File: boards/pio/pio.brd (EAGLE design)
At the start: 160 x 100 mm, 9 parts

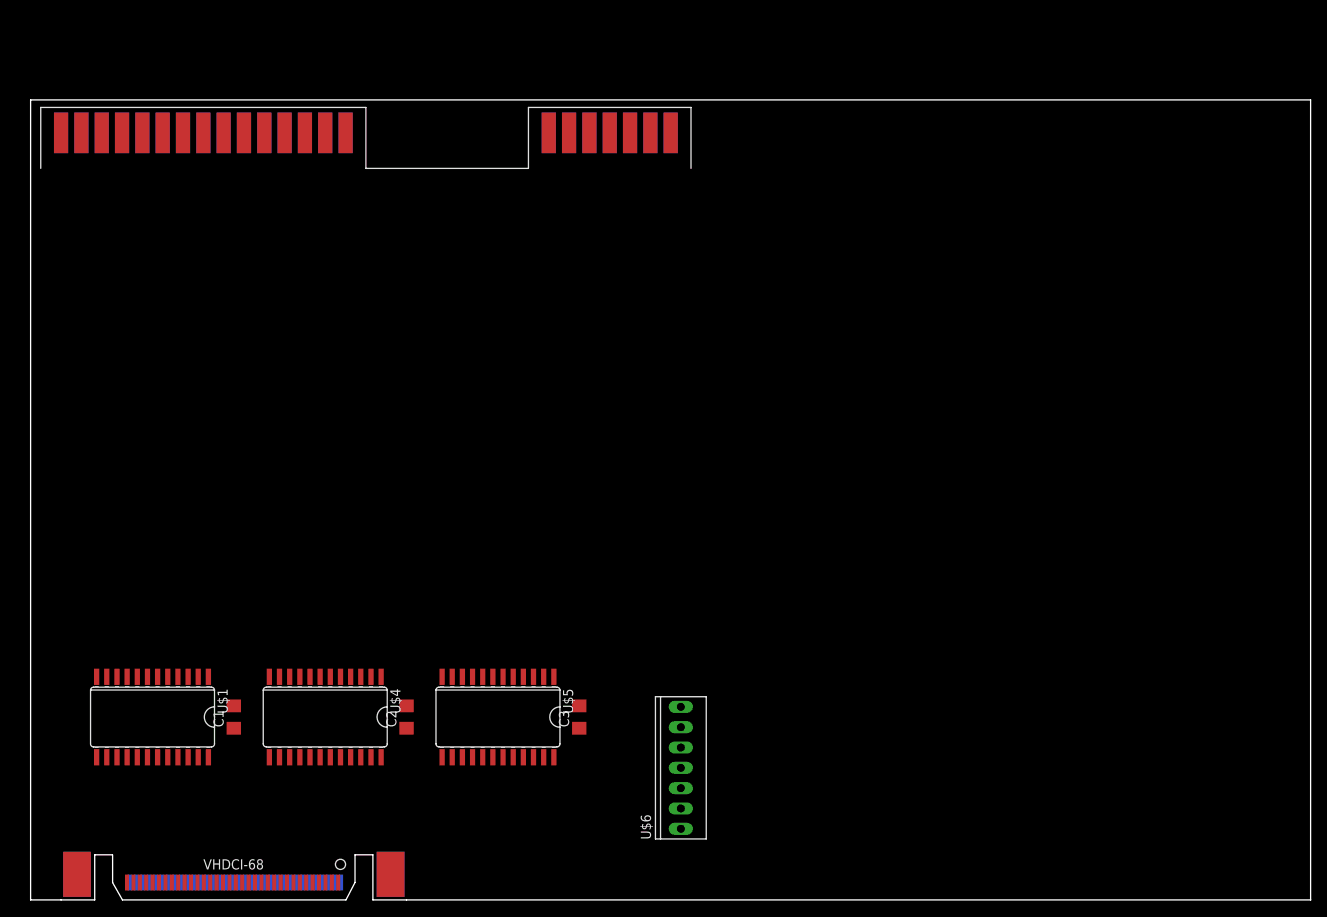
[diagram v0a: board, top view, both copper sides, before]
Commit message: Version of PIO to send off for manufacture
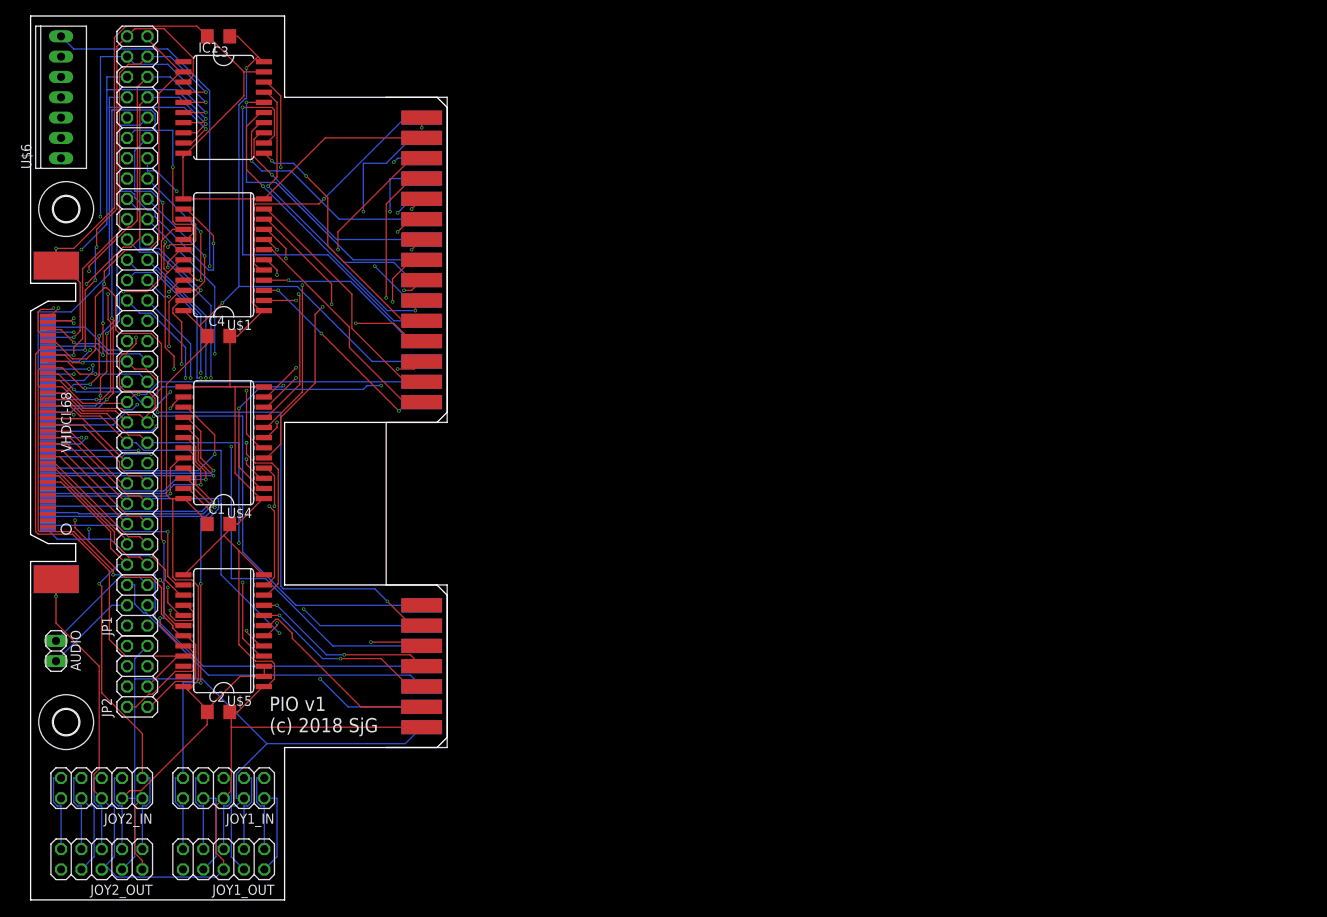
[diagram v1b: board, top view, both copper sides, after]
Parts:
- added AUDIO: (no value), pinhead:1X02
- added C4: 0.1uF, rcl:C1206
- added H1, H2: MOUNT-HOLE3.2, holes:3,2
- added IC1: 74AC245DW, 74xx-eu:SO20W
- added JOY1_IN, JOY1_OUT, JOY2_IN, JOY2_OUT: (no value), pinhead:2X05
- added JP1: (no value), pinhead:2X30
- added JP2: (no value), pinhead:2X04
- moved U$6 114.1 mm to (3.81, 100.3)
- moved C3 96.3 mm to (23.5, 108.0), turned to 180 degrees
- moved U$3 64.9 mm to (0.00, 59.7), turned to 270 degrees
- moved U$1 58.5 mm to (24.1, 80.6), turned to 90 degrees
- moved U$2 44.1 mm to (44.5, 100.3), turned to 270 degrees
- moved U$4 36.6 mm to (24.1, 57.1), turned to 90 degrees
- moved U$5 35.9 mm to (24.1, 33.7), turned to 90 degrees
- moved C1 24.2 mm to (23.5, 47.0), turned to 0 degrees
- moved C2 23.5 mm to (23.5, 23.5), turned to 0 degrees
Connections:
- removed net N$12: U$1.19, U$3.P53
- removed net N$13: U$1.20, U$3.P52
- removed net N$14: U$1.21, U$3.P51
- removed net N$15: U$1.14, U$3.P58
- removed net N$16: U$1.15, U$3.P57
- removed net N$17: U$1.16, U$3.P56
- removed net N$18: U$1.17, U$3.P55
- removed net N$19: U$1.18, U$3.P54
- removed net N$2: U$2.P$35, U$3.P68
- removed net N$20: U$1.22, U$3.P50
- removed net N$21: U$1.23, U$3.P49
- removed net N$32: U$3.P48, U$4.14
- removed net N$33: U$3.P47, U$4.15
- removed net N$34: U$3.P46, U$4.16
- removed net N$35: U$3.P45, U$4.17
- removed net N$36: U$3.P44, U$4.18
- removed net N$37: U$3.P43, U$4.19
- removed net N$38: U$3.P42, U$4.20
- removed net N$39: U$3.P41, U$4.21
- removed net N$40: U$3.P40, U$4.22
- removed net N$41: U$3.P39, U$4.23
- removed net N$50: U$3.P38, U$5.14
- removed net N$51: U$3.P37, U$5.15
- removed net N$52: U$3.P36, U$5.16
- removed net N$53: U$3.P35, U$5.17
- removed net N$54: U$3.P34, U$5.18
- removed net N$55: U$3.P33, U$5.19
- removed net N$56: U$3.P32, U$5.20
- removed net N$57: U$3.P31, U$5.21
- new net A0: JP1.44, U$1.23, U$3.P47
- new net A1: JP1.41, U$3.P46, U$4.14
- new net A10: JP1.34, U$3.P37, U$4.23
- new net A11: JP1.31, U$3.P36, U$5.14
- new net A12: JP1.32, U$3.P35, U$5.15
- new net A13: JP1.29, U$3.P34, U$5.16
- new net A14: JP1.30, U$3.P33, U$5.17
- new net A15: JP1.27, U$3.P32, U$5.18
- new net A2: JP1.42, U$3.P45, U$4.15
- new net A3: JP1.39, U$3.P44, U$4.16
- new net A4: JP1.40, U$3.P43, U$4.17
- new net A5: JP1.37, U$3.P42, U$4.18
- new net A6: JP1.38, U$3.P41, U$4.19
- new net A7: JP1.35, U$3.P40, U$4.20
- new net A8: JP1.36, U$3.P39, U$4.21
- new net A9: JP1.33, U$3.P38, U$4.22
- new net AUDIO: JP1.6, U$2.P$35, U$3.P66
- new net AUDIO_L: AUDIO.2, JP1.4, U$3.P67
- new net AUDIO_R: AUDIO.1, JP1.5, U$3.P68
- new net B02: JP1.47, U$1.18, U$3.P52
- new net CCTL: JP1.43, U$1.22, U$3.P48
- new net COMMAND: JP2.1, U$3.P31, U$5.19
- new net D0: IC1.2, JP1.59, U$3.P64
- new net D1: IC1.3, JP1.60, U$3.P63
- new net D1XX: JP1.50, U$1.17, U$3.P53
- new net D2: IC1.4, JP1.57, U$3.P62
- new net D3: IC1.5, JP1.58, U$3.P61
- new net D4: IC1.6, JP1.55, U$3.P60
- new net D5: IC1.7, JP1.56, U$3.P59
- new net D6: IC1.8, JP1.53, U$3.P58
- new net D7: IC1.9, JP1.54, U$3.P57
- new net DATA_OUT: JP2.2, U$3.P30, U$5.20
- new net G_IN0: JP1.3
- new net G_IN1: JP1.2
- new net G_IN2: JP1.1
- new net HALT: JP1.52, U$1.15, U$3.P55
- new net J1_1: JOY1_IN.1, JOY1_OUT.1, JP1.19, U$3.P21
- new net J1_2: JOY1_IN.2, JOY1_OUT.2, JP1.20, U$3.P20
- new net J1_3: JOY1_IN.3, JOY1_OUT.3, JP1.17, U$3.P19
- new net J1_4: JOY1_IN.5, JOY1_OUT.5, JP1.18, U$3.P18
- new net J1_5: JOY1_IN.7, JOY1_OUT.7, JP1.15, U$3.P17
- new net J1_A1: JOY1_IN.8, JOY1_OUT.8, JP1.16, U$3.P16
- new net J1_A2: JOY1_IN.9, JOY1_OUT.9, JP1.13, U$3.P15
- new net J2_1: JOY2_IN.1, JOY2_OUT.1, JP1.8, U$3.P8
- new net J2_2: JOY2_IN.2, JOY2_OUT.2, JP1.7, U$3.P9
- new net J2_3: JOY2_IN.3, JOY2_OUT.3, JP1.10, U$3.P10
- new net J2_4: JOY2_IN.5, JOY2_OUT.5, JP1.9, U$3.P11
- new net J2_5: JOY2_IN.7, JOY2_OUT.7, JP1.12, U$3.P12
- new net J2_A1: JOY2_IN.8, JOY2_OUT.8, JP1.11, U$3.P13
- new net J2_A2: JOY2_IN.9, JOY2_OUT.9, JP1.14, U$3.P14
- new net MTR_CTRL: JP2.3, U$3.P29, U$5.21
- new net N$67: IC1.11, U$2.P$11
- new net N$68: IC1.12, U$2.P$26
- new net N$69: IC1.13, U$2.P$22
- new net N$70: IC1.14, U$2.P$21
- new net N$71: IC1.15, U$2.P$10
- new net N$72: IC1.16, U$2.P$23
- new net N$73: IC1.17, U$2.P$24
- new net N$74: IC1.18, U$2.P$25
- new net REF: JP1.48, U$1.19, U$3.P51
- new net RST: JP1.49, U$1.16, U$3.P54
- new net RW: JP1.51, U$1.14, U$3.P56
- new net S4: JP1.45, U$1.20, U$3.P50
- new net S5: JP1.46, U$1.21, U$3.P49
- net !EXSEL!: now also JP1.25
- net !IRQ!: now also JP1.28, U$3.P28; no longer U$3.P26
- net !MPD!: now also JP1.26, U$3.P26; no longer U$3.P28
- net +5V: now also C4.1, IC1.20, JOY1_IN.4, JOY1_OUT.4, JOY2_IN.4, JOY2_OUT.4, JP2.7
- net GND: now also C4.2, IC1.10, IC1.19, JOY1_IN.6, JOY1_OUT.6, JOY2_IN.6, JOY2_OUT.6, U$3.P65; no longer U$3.P67
- net RD4: now also JP1.23, U$3.P25; no longer U$3.P30
- net RD5: now also JP1.24, U$3.P24; no longer U$3.P29
- net SIO_CLK_IN: now also JP1.22, U$3.P22; no longer U$3.P25
- net SIO_DATA_IN: now also JP1.21, U$3.P23; no longer U$3.P24
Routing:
- net GND: track 0.00 -> 329.3 mm, vias 0 -> 3
- net +5V: track 0.00 -> 251.3 mm, vias 0 -> 2
- net N$42: track 0.00 -> 93.0 mm, vias 0 -> 1
- net !MPD!: track 0.00 -> 91.2 mm, vias 0 -> 2
- net N$43: track 0.00 -> 86.1 mm, vias 0 -> 1
- net J1_2: track 0.00 -> 82.4 mm, vias 0 -> 1
- net DATA_OUT: track 0.00 -> 81.8 mm, vias 0 -> 2
- net AUDIO: track 0.00 -> 81.5 mm, vias 0 -> 1
- net N$44: track 0.00 -> 80.8 mm, vias 0 -> 1
- net J1_1: track 0.00 -> 79.9 mm, vias 0 -> 1
- net SIO_CLK_IN: track 0.00 -> 79.4 mm, vias 0 -> 1
- net !IRQ!: track 0.00 -> 76.0 mm, vias 0 -> 3
- net D1XX: track 0.00 -> 75.2 mm, vias 0 -> 3
- net N$3: track 0.00 -> 74.9 mm, vias 0 -> 2
- net J1_A2: track 0.00 -> 74.2 mm, vias 0 -> 2
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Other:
- board size 160 x 100 mm -> 52.1 x 110.5 mm
- board text added: "PIO v1 (c) 2018 SjG"

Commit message: Ok, belay that last. *This* is the one to go to the fab.
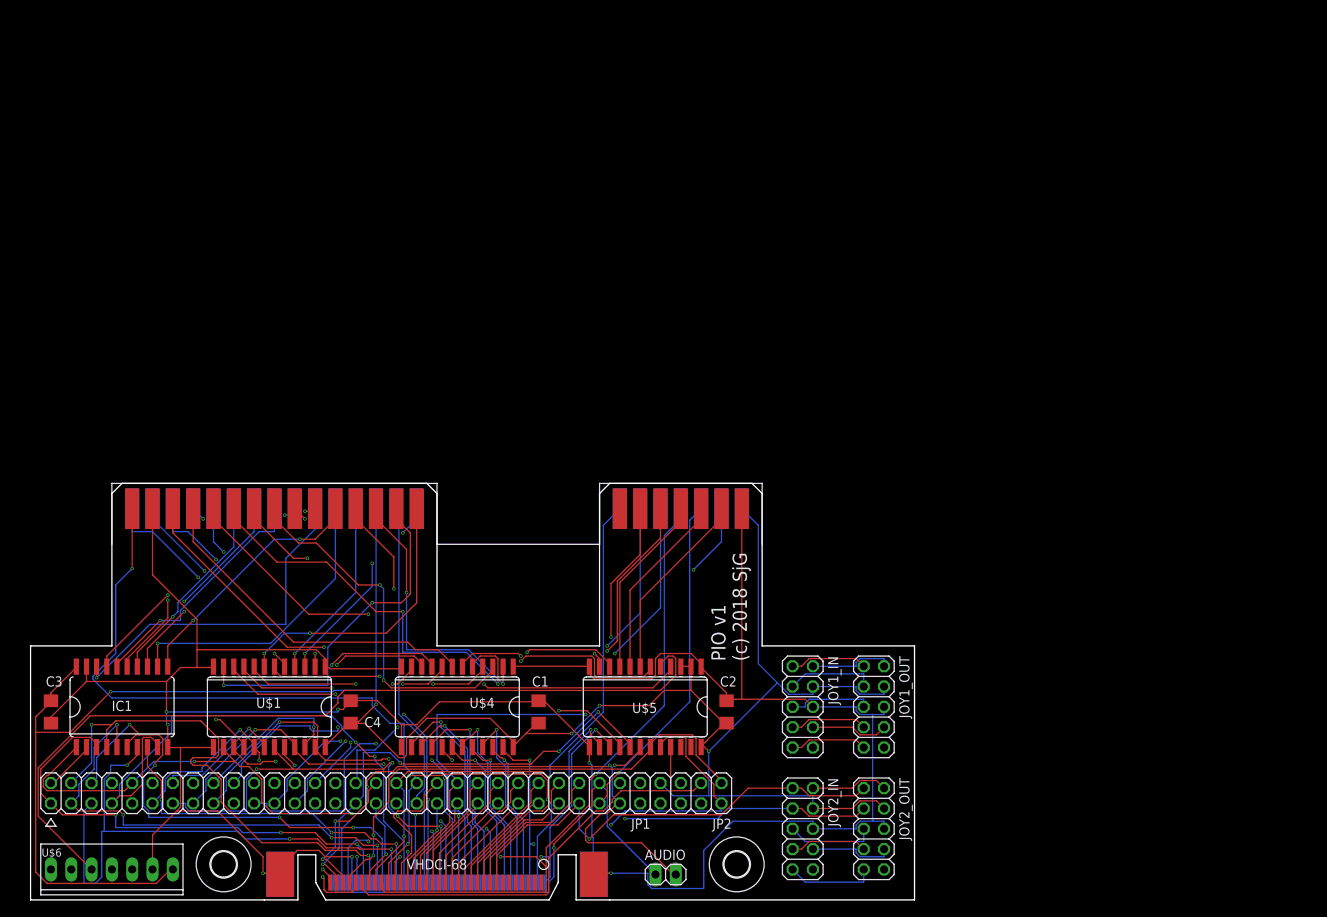
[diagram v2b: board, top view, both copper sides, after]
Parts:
- moved U$6 96.7 mm to (10.2, 3.81), turned to 180 degrees
- moved JOY2_OUT 96.6 mm to (105.4, 8.89), turned to 270 degrees
- moved JOY2_IN 87.8 mm to (96.5, 8.89), turned to 270 degrees
- moved C3 87.0 mm to (2.54, 23.5), turned to 270 degrees
- moved H1 85.7 mm to (88.3, 4.45), turned to 90 degrees
- moved H2 84.2 mm to (24.1, 4.45), turned to 90 degrees
- moved JOY1_OUT 83.5 mm to (105.4, 24.1), turned to 270 degrees
- moved AUDIO 81.2 mm to (79.4, 3.17), turned to 0 degrees
- moved U$3 78.4 mm to (50.8, 0.00), turned to 0 degrees
- moved IC1 76.0 mm to (11.4, 24.1), turned to 0 degrees
- moved JOY1_IN 73.1 mm to (96.5, 24.1), turned to 270 degrees
- moved JP2 70.7 mm to (82.5, 13.3), turned to 180 degrees
- moved U$2 65.6 mm to (10.2, 44.5), turned to 0 degrees
- moved JP1 64.0 mm to (38.1, 13.3), turned to 180 degrees
- moved C2 63.5 mm to (87.0, 23.5), turned to 90 degrees
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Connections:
- net +5V: now also U$6.1
- net GND: now also U$6.2
- net RW: now also IC1.1
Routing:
- net +5V: track 251.3 -> 284.1 mm, vias 2 -> 5
- net GND: track 329.3 -> 359.5 mm, vias 3 -> 7
- net D1XX: track 75.2 -> 54.7 mm
- net N$43: track 86.1 -> 105.3 mm, vias 1 -> 0
- net A15: track 49.7 -> 67.9 mm, vias 2 -> 3
- net N$68: track 53.2 -> 37.2 mm
- net RD4: track 72.5 -> 87.1 mm, vias 3 -> 2
- net N$28: track 39.1 -> 53.1 mm
- net N$27: track 41.3 -> 55.1 mm
- net N$1: track 31.2 -> 44.6 mm, vias 0 -> 2
- net J1_A2: track 74.2 -> 61.9 mm, vias 2 -> 0
- net D5: track 61.6 -> 73.4 mm
- net AUDIO_L: track 59.3 -> 70.7 mm, vias 1 -> 2
- net RST: track 51.5 -> 62.6 mm, vias 4 -> 2
- net A4: track 64.1 -> 53.2 mm, vias 2 -> 3
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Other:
- board size 52.1 x 110.5 mm -> 110.5 x 52.1 mm
